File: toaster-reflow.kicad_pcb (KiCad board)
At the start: 2 copper layers, 40.1 x 51.8 mm, 41 parts, among them J1 1935161, J2 1935161, J3 Raspberry_Pi_2_3, J4 Conn_01x04, J6 Conn_01x03, K1 1-1415899-3, Q1 Q_NMOS_GSD, Q2 Q_NMOS_GSD, Q3 Q_PNP_BEC, Q4 Q_PNP_BEC, U1 3.3V Ref, U2 MAX31856, U3 MAX31856

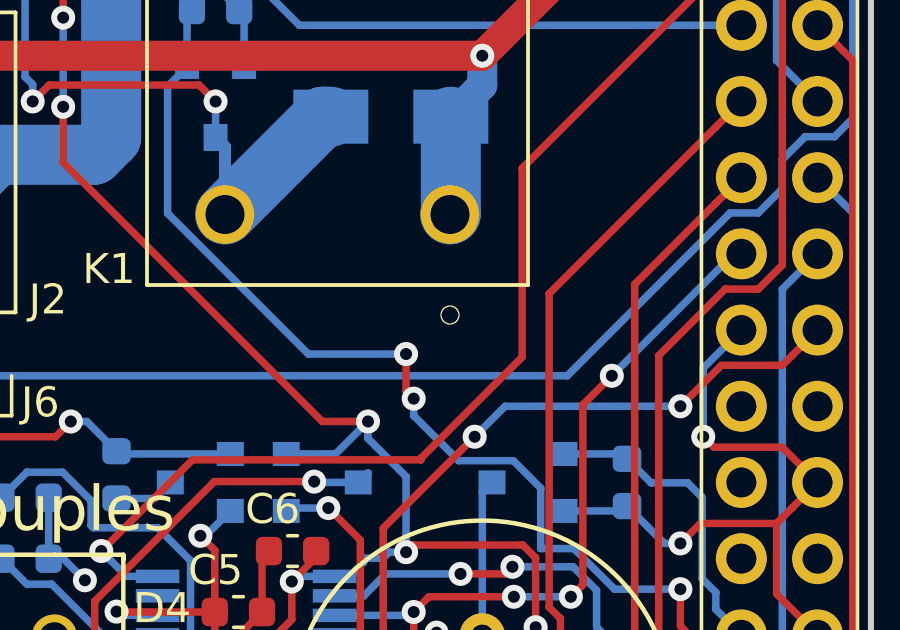
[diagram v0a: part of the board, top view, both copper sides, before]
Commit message: update some stuff
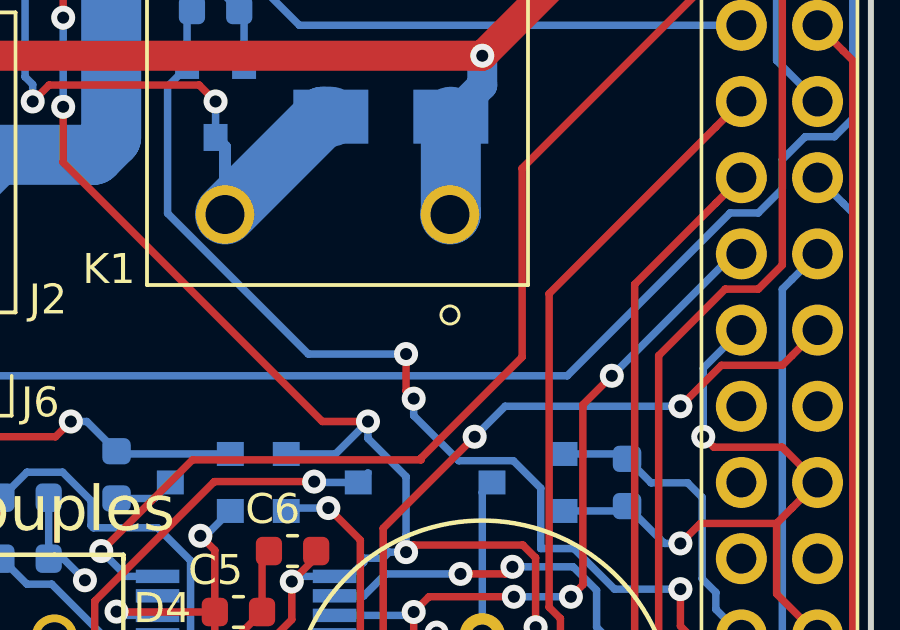
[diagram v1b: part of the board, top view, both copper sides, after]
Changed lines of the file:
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@@
-(kicad_pcb (version 20171130) (host pcbnew 5.0.0)
+(kicad_pcb (version 20171130) (host pcbnew 5.0.1)
   (general
     (thickness 1.6)
@@
     (pad_drill 0.762)
     (pad_to_mask_clearance 0.2)
+    (solder_mask_min_width 0.25)
     (aux_axis_origin 0 0)
     (visible_elements FFFFFF7F)
     (pcbplotparams
-      (layerselection 0x010fc_ffffffff)
+      (layerselection 0x010ff_ffffffff)
       (usegerberextensions false)
       (usegerberattributes false)
@@
       (outputformat 1)
       (mirror false)
-      (drillshape 1)
+      (drillshape 0)
       (scaleselection 1)
-      (outputdirectory ""))
+      (outputdirectory "gerbers"))
   )
   (net 0 "")
@@
       (effects (font (size 1.00198 1.00198) (thickness 0.05)))
     )
-    (fp_circle (center -15.5 3.75) (end -15.2 3.75) (layer F.SilkS) (width 0))
+    (fp_circle (center -15.5 3.75) (end -15.2 3.75) (layer F.SilkS) (width 0.1))
     (fp_line (start -14.75 6.6) (end -14.75 -6.6) (layer Eco1.User) (width 0.05))
     (fp_line (start 14.75 6.6) (end -14.75 6.6) (layer Eco1.User) (width 0.05))
@@
     (pad 1 thru_hole rect (at 0 0) (size 1.7 1.7) (drill 1) (layers *.Cu *.Mask)
       (net 6 +3V3))
-    (model ${KISYS3DMOD}/Connector_PinHeader_2.54mm.3dshapes/PinHeader_2x20_P2.54mm_Vertical.wrl
-      (at (xyz 0 0 0))
-      (scale (xyz 1 1 1))
-      (rotate (xyz 0 0 0))
-    )
     (model ${KIPRJMOD}/kicad-packages3D/Connector_PinSocket_2.54mm.3dshapes/PinSocket_2x20_P2.54mm_Vertical.wrl
       (offset (xyz 0 0 -1.6))
@@
   (segment (start 123.6725 120.091) (end 123.6725 119.634) (width 0.25) (layer B.Cu) (net 8) (status 30))
   (segment (start 125.222 121.6405) (end 123.6725 120.091) (width 0.25) (layer B.Cu) (net 8) (status 30))
-  (segment (start 137.512 122.712) (end 136.622 122.712) (width 0.25) (layer B.Cu) (net 46) (status 10))
   (segment (start 137.471888 122.102112) (end 137.512 122.062) (width 0.25) (layer B.Cu) (net 8) (status 30))
   (segment (start 132.287612 122.102112) (end 137.471888 122.102112) (width 0.25) (layer B.Cu) (net 8) (status 20))
   (segment (start 131.826 121.6405) (end 132.287612 122.102112) (width 0.25) (layer B.Cu) (net 8) (status 10))
-  (segment (start 135.606 122.712) (end 137.512 122.712) (width 0.25) (layer B.Cu) (net 46) (status 20))
-  (segment (start 134.030999 124.287001) (end 135.606 122.712) (width 0.25) (layer B.Cu) (net 46))
   (segment (start 127.0255 88.9) (end 130.7845 88.9) (width 0.25) (layer F.Cu) (net 9) (status 30))
   (segment (start 144.526 110.166) (end 144.202 110.49) (width 0.25) (layer B.Cu) (net 10) (status 30))
@@
   (segment (start 133.35 97.224315) (end 133.096 96.970315) (width 0.25) (layer B.Cu) (net 45))
   (segment (start 133.35 97.79) (end 133.35 97.224315) (width 0.25) (layer B.Cu) (net 45))
+  (segment (start 137.512 122.712) (end 136.622 122.712) (width 0.25) (layer B.Cu) (net 46) (status 10))
+  (segment (start 135.606 122.712) (end 137.512 122.712) (width 0.25) (layer B.Cu) (net 46) (status 20))
+  (segment (start 134.030999 124.287001) (end 135.606 122.712) (width 0.25) (layer B.Cu) (net 46))
   (segment (start 125.2875 123.15) (end 125.222 123.2155) (width 0.25) (layer B.Cu) (net 46) (status 30))
   (segment (start 129.072 123.15) (end 125.2875 123.15) (width 0.25) (layer B.Cu) (net 46) (status 30))
